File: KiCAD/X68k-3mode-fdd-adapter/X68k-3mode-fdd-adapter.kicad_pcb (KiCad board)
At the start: 2 copper layers, 53 x 72 mm, 50 parts, among them J1 Conn_02x17_Odd_Even, J2 Conn_02x17_Odd_Even, J3 Conn_01x04, J4 Conn_01x04, J5 Conn_01x02_Pin, J6 Conn_01x04, J7 Conn_01x05_Pin, J8 Conn_01x05_Pin, Q1 2SC4213, SW1 SW_DIP_x04, U1 CH32V003F4U6, U2 74HC14, U3 74HC14, U4 74HC153, U5 74HC153, U6 ULN2003A

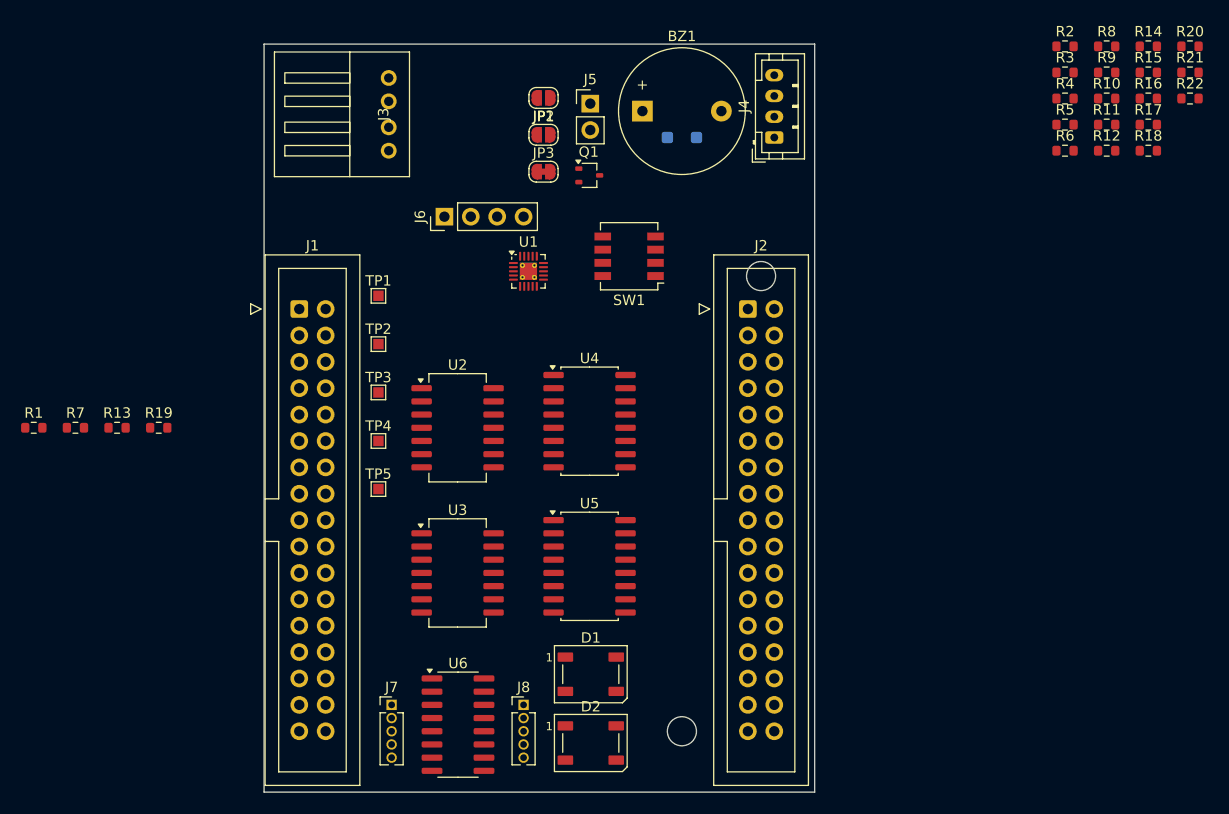
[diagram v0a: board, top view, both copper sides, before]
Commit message: 一通り配線した(未チェック)
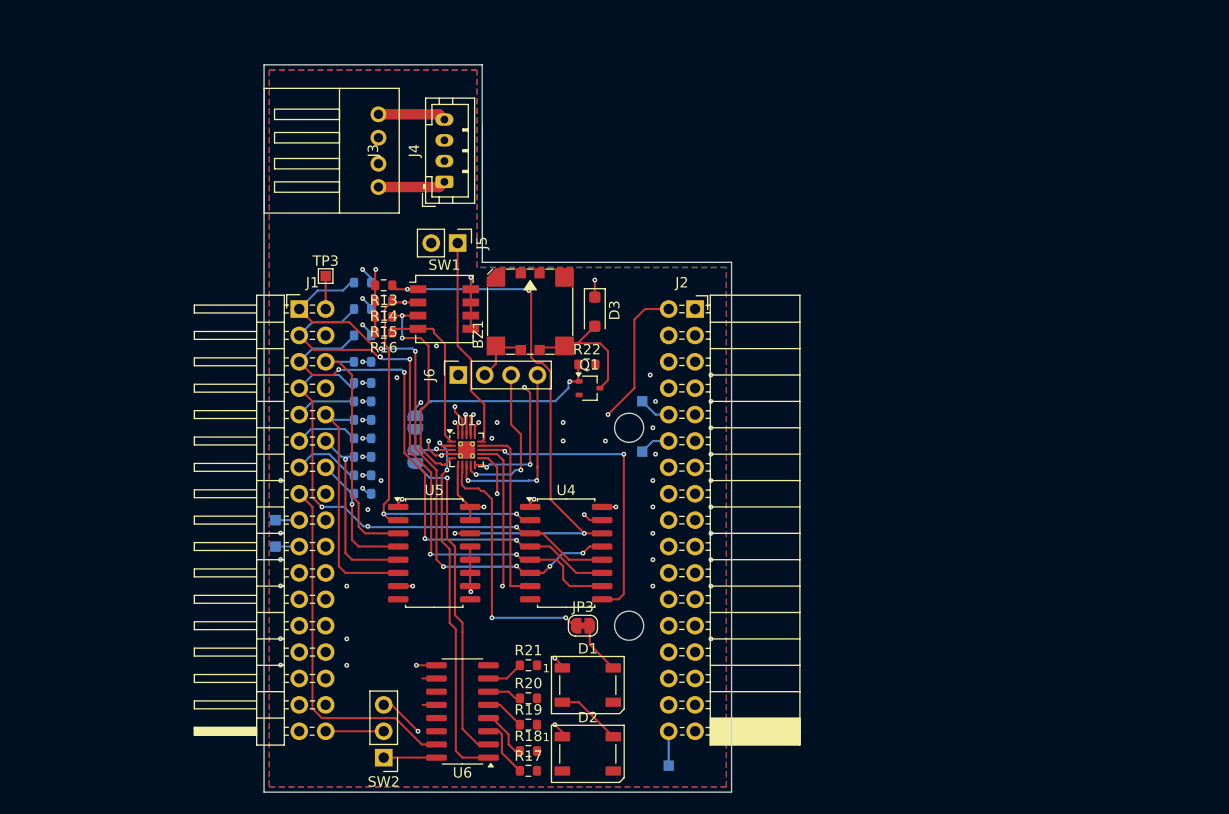
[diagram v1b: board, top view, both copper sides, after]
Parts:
- removed J7, J8: Conn_01x05_Pin, Connector_PinHeader_1.27mm:PinHeader_1x05_P1.27mm_Vertical
- removed R11: 1K, Resistor_SMD:R_0603_1608Metric
- removed U2, U3: 74HC14, Package_SO:SO-14_5.3x10.2mm_P1.27mm
- added SW2: SW_SPDT, Connector_PinHeader_2.54mm:PinHeader_1x03_P2.54mm_Vertical, F.Cu at (80.5, 106.7)
- added TP6: TestPoint, TestPoint:TestPoint_Pad_1.0x1.0mm, B.Cu at (108.0, 107.4)
- BZ1: footprint Buzzer_Beeper:Buzzer_12x9.5RM7.6 -> x68k-lib:UGCT7525AN4
- D3: moved to F.Cu
- J1: footprint Connector_IDC:IDC-Header_2x17_P2.54mm_Vertical -> x68k-lib:PinHeader_2x17_P2.54mm_Horizontal_Mirror
- J2: footprint Connector_IDC:IDC-Header_2x17_P2.54mm_Vertical -> x68k-lib:PinSocket_2x17_P2.54mm_Horizontal_Mirror
- J6: footprint Connector_PinHeader_2.54mm:PinHeader_1x04_P2.54mm_Vertical -> Connector_PinSocket_2.54mm:PinSocket_1x04_P2.54mm_Vertical
- JP1, JP2, R1, R10, R12, R2, R3, R4, R5, R6, R7, R8, R9, TP1, TP2, TP4, TP5: moved to B.Cu
- moved R20 89.4 mm to (94.4, 101.0)
- moved R17 86.2 mm to (94.4, 108.0)
- moved R21 85.5 mm to (94.4, 97.8)
- moved R8 83.6 mm to (78.5, 81.3), turned to 180 degrees
- moved R18 83.1 mm to (94.4, 106.0)
- moved R9 79.8 mm to (78.5, 75.9), turned to 180 degrees
- moved R12 78.1 mm to (78.5, 79.5), turned to 180 degrees
- moved R14 77.6 mm to (80.5, 62.7), turned to 180 degrees
- moved R10 77.3 mm to (78.5, 72.4), turned to 180 degrees
- moved R15 77.3 mm to (80.5, 64.3), turned to 180 degrees
- moved R16 77.0 mm to (80.5, 65.8), turned to 180 degrees
- moved R4 72.9 mm to (78.5, 70.6), turned to 180 degrees
- moved R6 72.4 mm to (78.5, 74.2), turned to 180 degrees
- moved R3 72.2 mm to (78.5, 66.0), turned to 180 degrees
- moved R2 72.2 mm to (78.5, 63.5), turned to 180 degrees
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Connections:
- net /OPTION_SELECT_MAIN renamed /OPTION_SELECT
- net /OPTION_SELECT_SUB renamed /OPTION_SELECT_PAIR
- J2 pad 34: /READY -> /DISK_CHANGE
- U1 pad 18: /EJECT_MASK_BUF -> /EJECT_MASK
- U1 pad 19: /EJECT_BUF -> /EJECT
- U1 pad 20: /LED_BLINK_BUF -> /LED_BLINK
- U4 pad 10: /OPTION_SELECT_1_BUF -> /OPTION_SELECT_1
- U4 pad 11: /OPTION_SELECT_2_BUF -> /OPTION_SELECT_2
- U4 pad 12: /OPTION_SELECT_3_BUF -> /OPTION_SELECT_3
- U4 pad 13: /OPTION_SELECT_0_BUF -> /OPTION_SELECT_0
- U4 pad 3: /OPTION_SELECT_3_BUF -> /OPTION_SELECT_3
- U4 pad 4: /OPTION_SELECT_2_BUF -> /OPTION_SELECT_2
- U4 pad 5: /OPTION_SELECT_1_BUF -> /OPTION_SELECT_1
- U4 pad 6: /OPTION_SELECT_0_BUF -> /OPTION_SELECT_0
- U5 pad 3: /DRIVE_SELECT_3_BUF -> /DRIVE_SELECT_3
- U5 pad 4: /DRIVE_SELECT_2_BUF -> /DRIVE_SELECT_2
- U5 pad 5: /DRIVE_SELECT_1_BUF -> /DRIVE_SELECT_1
- U5 pad 6: /DRIVE_SELECT_0_BUF -> /DRIVE_SELECT_0
- U6 pad 10: Net-(J8-Pin_5) -> unconnected-(U6-O7-Pad10)
- U6 pad 11: Net-(J8-Pin_4) -> unconnected-(U6-O6-Pad11)
- U6 pad 12: Net-(J8-Pin_3) -> unconnected-(U6-O5-Pad12)
- U6 pad 13: Net-(J8-Pin_2) -> unconnected-(U6-O4-Pad13)
- U6 pad 14: Net-(J8-Pin_1) -> unconnected-(U6-O3-Pad14)
- U6 pad 16: /READY -> /READY_GEN_BUF
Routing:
- net GND: track 0.00 -> 122.1 mm, vias 0 -> 44
- net /OPTION_SELECT_0: track 0.00 -> 57.7 mm, vias 0 -> 6
- net /OPTION_SELECT_1: track 0.00 -> 56.1 mm, vias 0 -> 5
- net /DIPSW_0: track 0.00 -> 56.0 mm, vias 0 -> 4
- net /OPTION_SELECT_2: track 0.00 -> 52.6 mm, vias 0 -> 4
- net /OPTION_SELECT_3: track 0.00 -> 47.7 mm, vias 0 -> 3
- net /INDEX: track 0.00 -> 46.2 mm, vias 0 -> 3
- net +5V: track 0.00 -> 43.4 mm, vias 0 -> 18
- net /DIPSW_1: track 0.00 -> 39.7 mm, vias 0 -> 3
- net /MOTOR_ON: track 0.00 -> 37.4 mm, vias 0 -> 1
- net /READY_GEN: track 0.00 -> 37.0 mm, vias 0 -> 2
- net /TRACK_00: track 0.00 -> 34.7 mm
- net /DISK_IN: track 0.00 -> 34.6 mm
- net /SIDE_SELECT: track 0.00 -> 34.1 mm
- net /WRITE_PROTECT: track 0.00 -> 33.0 mm
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- added copper zone on In1.Cu, net +5V
- added copper zone on B.Cu, net GND
- added copper zone on F.Cu, net GND
- added copper zone on In2.Cu, net GND
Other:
- board size 53 x 72 mm -> 45 x 70 mm
- copper layers 2 -> 4
